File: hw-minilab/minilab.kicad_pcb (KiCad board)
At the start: 2 copper layers, 165 x 60 mm, 67 parts, among them J1 Screw_Terminal_01x02, J10 Screw_Terminal_01x03, J11 Screw_Terminal_01x03, J12 Conn_01x09_Male, J2 Screw_Terminal_01x02, J3 Conn_01x09_Male, J4 Screw_Terminal_01x04, J5 Screw_Terminal_01x03, J6 Screw_Terminal_01x03, J7 Screw_Terminal_01x03, J8 Screw_Terminal_01x03, J9 Screw_Terminal_01x03, SW1 SW_DPDT_x2, SW2 SW_SPDT, U1 NE555P, U2 L7805, U3 KF33, U4 4069, U5 4069

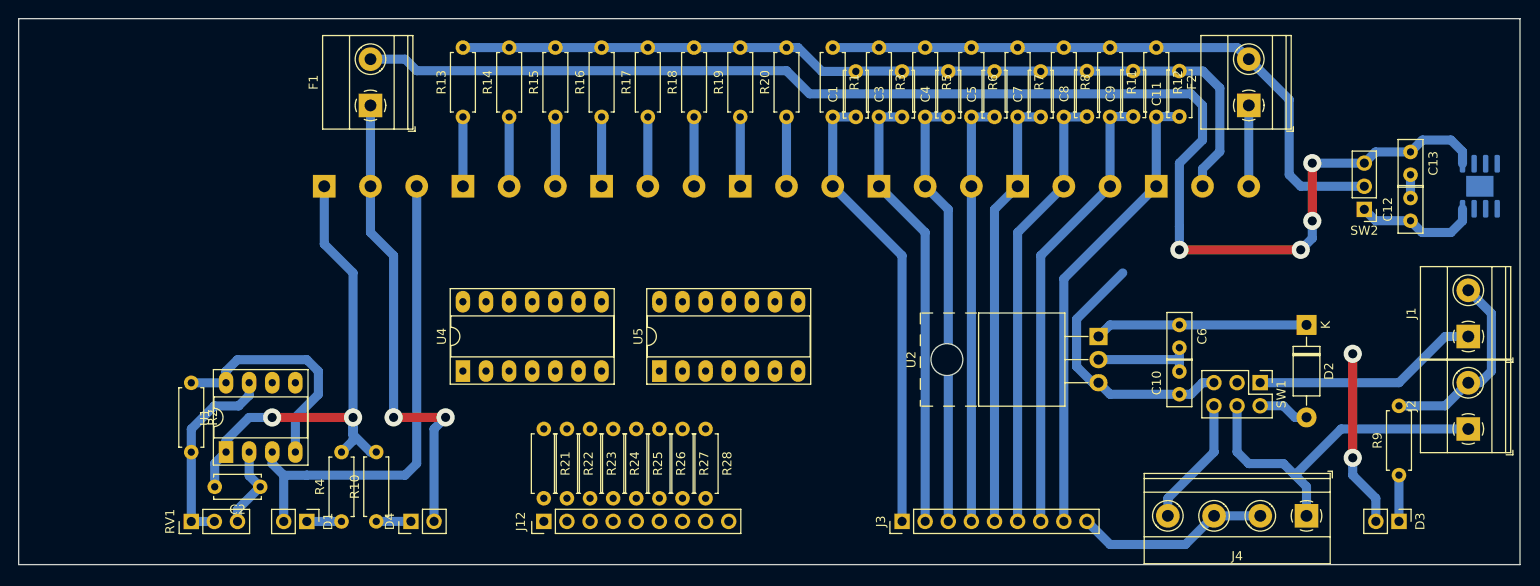
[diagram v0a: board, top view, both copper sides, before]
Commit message: Archivos de fabricacion generados
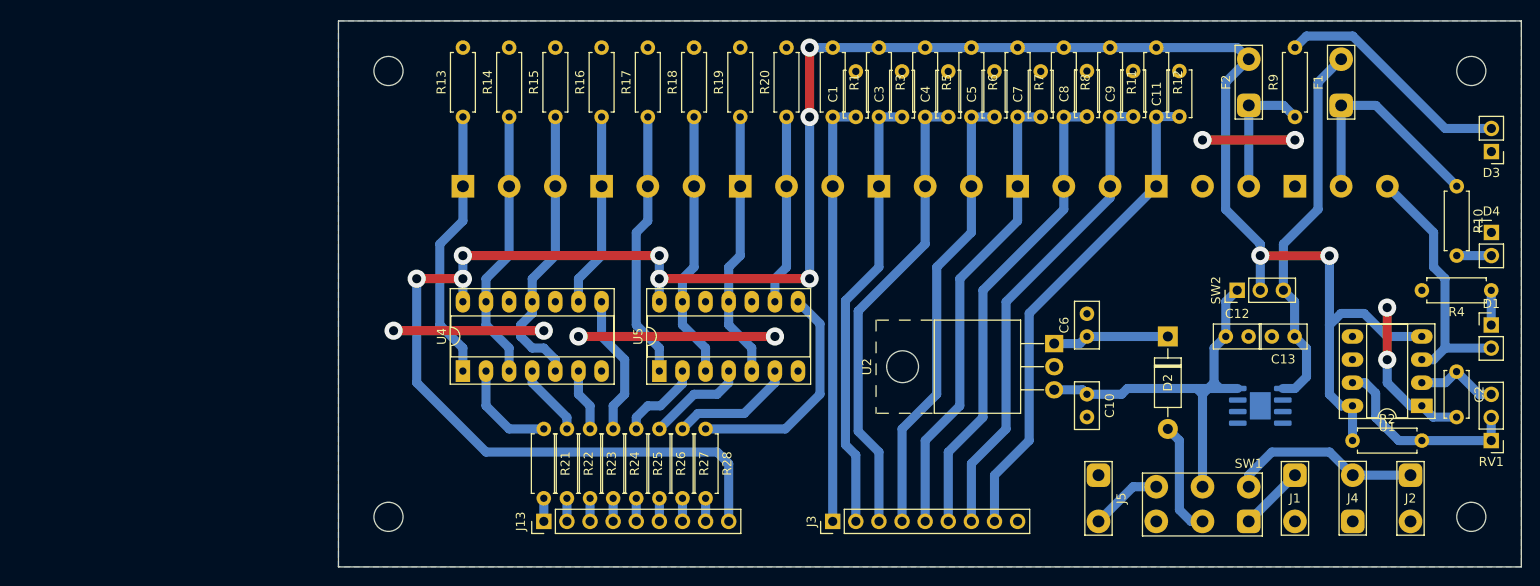
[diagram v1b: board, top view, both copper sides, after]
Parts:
- added H1: MountingHole, MountingHole:MountingHole_3.2mm_M3, F.Cu at (217.5, 126.5)
- added H2: MountingHole, MountingHole:MountingHole_3.2mm_M3, F.Cu at (98.5, 126.5)
- added H3: MountingHole, MountingHole:MountingHole_3.2mm_M3, F.Cu at (98.5, 77.5)
- added H4: MountingHole, MountingHole:MountingHole_3.2mm_M3, F.Cu at (217.5, 77.5)
- added J5: Screw_Terminal_01x02, TestPoint:TestPoint_2Pads_Pitch5.08mm_Drill1.3mm, F.Cu at (176.5, 121.9)
- F1, F2, J1, J2: footprint TerminalBlock_Phoenix:TerminalBlock_Phoenix_MKDS-1,5-2-5.08_1x02_P5.08mm_Horizontal -> TestPoint:TestPoint_2Pads_Pitch5.08mm_Drill1.3mm
- J4: value Screw_Terminal_01x04 -> Screw_Terminal_01x02; footprint TerminalBlock_Phoenix:TerminalBlock_Phoenix_MKDS-1,5-4-5.08_1x04_P5.08mm_Horizontal -> TestPoint:TestPoint_2Pads_Pitch5.08mm_Drill1.3mm
- SW1: footprint Connector_PinHeader_2.54mm:PinHeader_2x03_P2.54mm_Vertical -> Library:TestPoint_6Pads_Pitch5.08mm_Drill1.3mm
- moved RV1 143.1 mm to (219.7, 118.1), turned to 180 degrees
- moved C2 132.1 mm to (215.9, 110.5), turned to -90 degrees
- moved D1 131.9 mm to (219.7, 105.4), turned to 0 degrees
- moved U1 131.5 mm to (212.1, 114.3), turned to 180 degrees
- moved R4 128.9 mm to (219.7, 101.6), turned to 180 degrees
- moved R2 127.8 mm to (204.4, 118.1), turned to 0 degrees
- moved R10 124.3 mm to (215.9, 90.2), turned to -90 degrees
- moved D4 122.9 mm to (219.7, 95.2), turned to 0 degrees
- moved J6 106.7 mm to (198.1, 90.2)
- moved F1 106.7 mm to (203.2, 81.3)
- moved D3 41.9 mm to (219.7, 86.4), turned to 180 degrees
- moved R9 41.0 mm to (198.1, 82.5)
- moved U3 34.1 mm to (194.3, 114.3), turned to 180 degrees
- moved J1 24.4 mm to (198.1, 121.9), turned to -90 degrees
- moved C12 24.0 mm to (190.5, 106.7), turned to 0 degrees
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- renumbered J9 to J10, J10 to J11, J11 to J12, J12 to J13, J5 to J6, J6 to J7, J7 to J8, J8 to J9
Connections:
- D3 pad 1: Net-(D3-Pad1) -> GND
- D4 pad 1: Net-(D4-Pad1) -> GND
- F1 pad 1: Net-(D4-Pad2) -> Net-(F1-Pad1)
- F2 pad 1: Net-(D3-Pad2) -> Net-(F2-Pad1)
- J4 pad 1: Net-(J2-Pad1) -> GND
- J4 pad 2: GND -> Net-(J2-Pad1)
- J6 pad 2: Net-(D4-Pad2) -> Net-(F1-Pad1)
- J7 pad 3: Net-(D3-Pad2) -> Net-(F2-Pad1)
- R10 pad 1: Net-(D4-Pad1) -> Net-(F1-Pad1)
- R10 pad 2: GND -> Net-(D4-Pad2)
- R9 pad 1: Net-(D3-Pad1) -> Net-(F2-Pad1)
- R9 pad 2: GND -> Net-(D3-Pad2)
- SW1 pad 6: Net-(J4-Pad4) -> Net-(J5-Pad2)
- U3 pad 2: (no net) -> GND
- U3 pad 3: (no net) -> GND
- U3 pad 6: (no net) -> GND
- U3 pad 7: (no net) -> GND
- U3 pad 9: (no net) -> GND
- U4 pad 10: Net-(R25-Pad1) -> unconnected-(U4-Pad10)
- U4 pad 11: /IN4 -> /IN2
- U4 pad 12: Net-(R26-Pad1) -> unconnected-(U4-Pad12)
- U4 pad 13: /IN5 -> /IN1
- U5 pad 1: /IN6 -> /IN4
- U5 pad 10: (no net) -> unconnected-(U5-Pad10)
- U5 pad 11: (no net) -> /IN6
- U5 pad 12: (no net) -> unconnected-(U5-Pad12)
- U5 pad 13: (no net) -> /IN5
- U5 pad 2: Net-(R27-Pad1) -> Net-(R25-Pad1)
- U5 pad 3: /IN7 -> /IN5
- U5 pad 4: Net-(R28-Pad1) -> Net-(R26-Pad1)
- U5 pad 5: (no net) -> /IN6
- U5 pad 6: (no net) -> Net-(R27-Pad1)
- U5 pad 8: (no net) -> Net-(R28-Pad1)
- U5 pad 9: (no net) -> /IN7
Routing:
- net VCC: track 95.8 -> 252.8 mm, vias 0 -> 10
- net GND: track 210.7 -> 65.8 mm, vias 2 -> 8
- net +3V3: track 153.3 -> 41.7 mm, vias 4 -> 0
- net Net-(D4-Pad2): track 53.0 -> 3.81 mm, vias 2 -> 0
- net Net-(R28-Pad1): track 0.00 -> 25.3 mm
- net Net-(F1-Pad1): track 0.00 -> 25.3 mm
- net /OSC: track 53.8 -> 28.6 mm
- net /IN2: track 7.62 -> 31.8 mm
- net /IN1: track 7.62 -> 30.0 mm
- net /IN0: track 7.62 -> 30.0 mm
- net /IN6: track 7.62 -> 29.5 mm
- net /IN5: track 7.62 -> 29.5 mm
- net /IN4: track 7.62 -> 29.5 mm
- net Net-(J1-Pad1): track 25.0 -> 7.18 mm
- net Net-(J2-Pad1): track 38.6 -> 21.2 mm
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- added copper zone on B.Cu, net GND
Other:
- board size 165 x 60 mm -> 130 x 60 mm
